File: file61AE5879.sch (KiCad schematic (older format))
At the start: 10 parts, among them U1 8086_Min_Mode, U2 74LS245, U3 74LS245, U4 74LS373, U5 74LS373, U6 74LS373

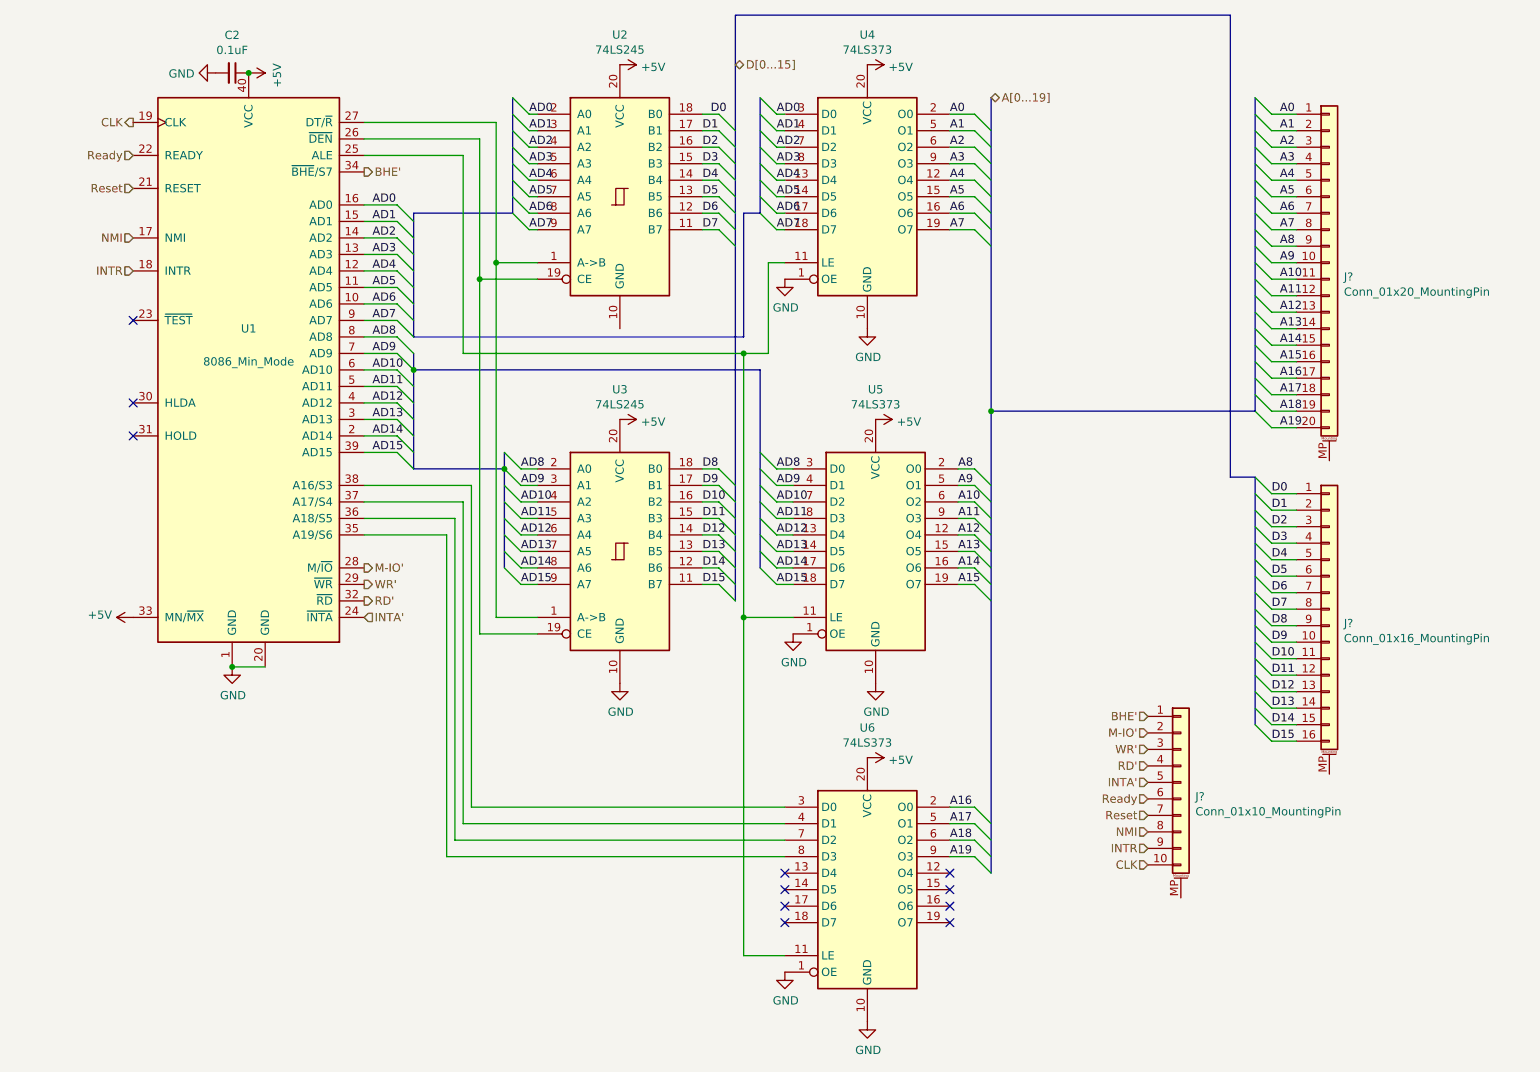
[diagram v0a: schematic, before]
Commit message: Fixing Weirdness
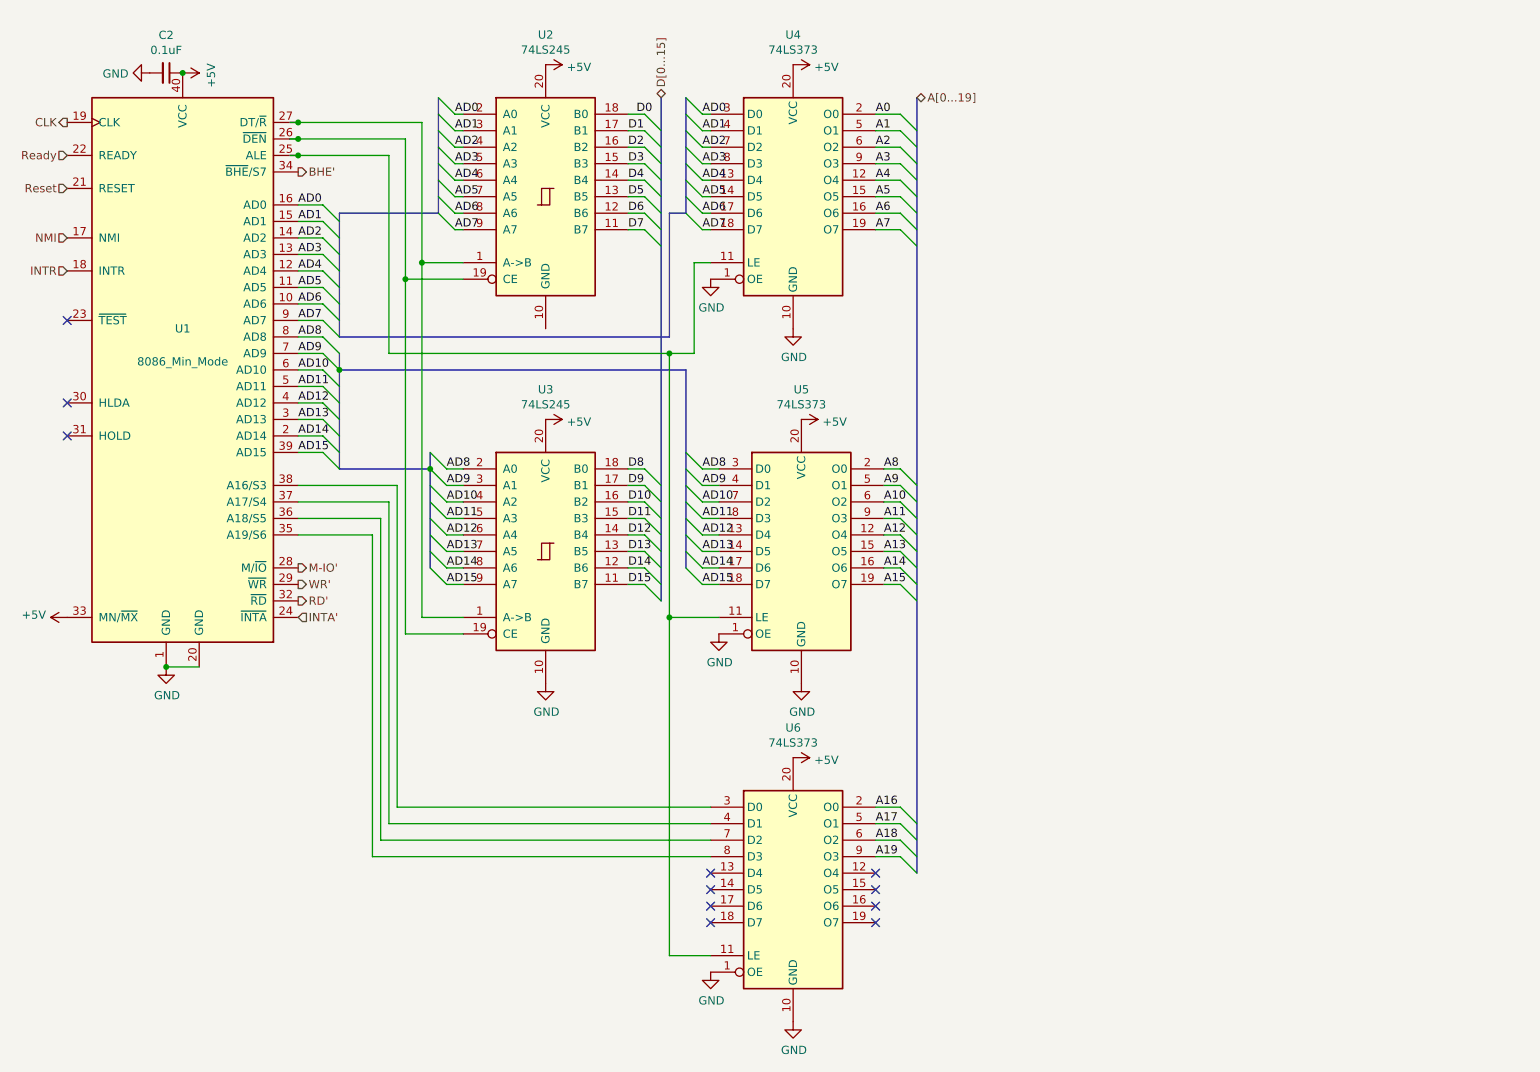
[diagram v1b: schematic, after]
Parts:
- removed J?: Conn_01x20_MountingPin, symbol Connector_Generic_MountingPin:Conn_01x20_MountingPin
- removed J?: Conn_01x16_MountingPin, symbol Connector_Generic_MountingPin:Conn_01x16_MountingPin
- removed J?: Conn_01x10_MountingPin, symbol Connector_Generic_MountingPin:Conn_01x10_MountingPin
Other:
- moved on the sheet: C2, U1, U2, U3, U4, U5, U6
